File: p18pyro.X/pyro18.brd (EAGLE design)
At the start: 74.9 x 46.7 mm, 25 parts, among them U1 TPIC6B595PTH, U2 TPIC6B595PTH, X1 332-10, X2 332-10, X3 332-10, X4 332-10, X5 22-23-2041, X7 22-23-2021

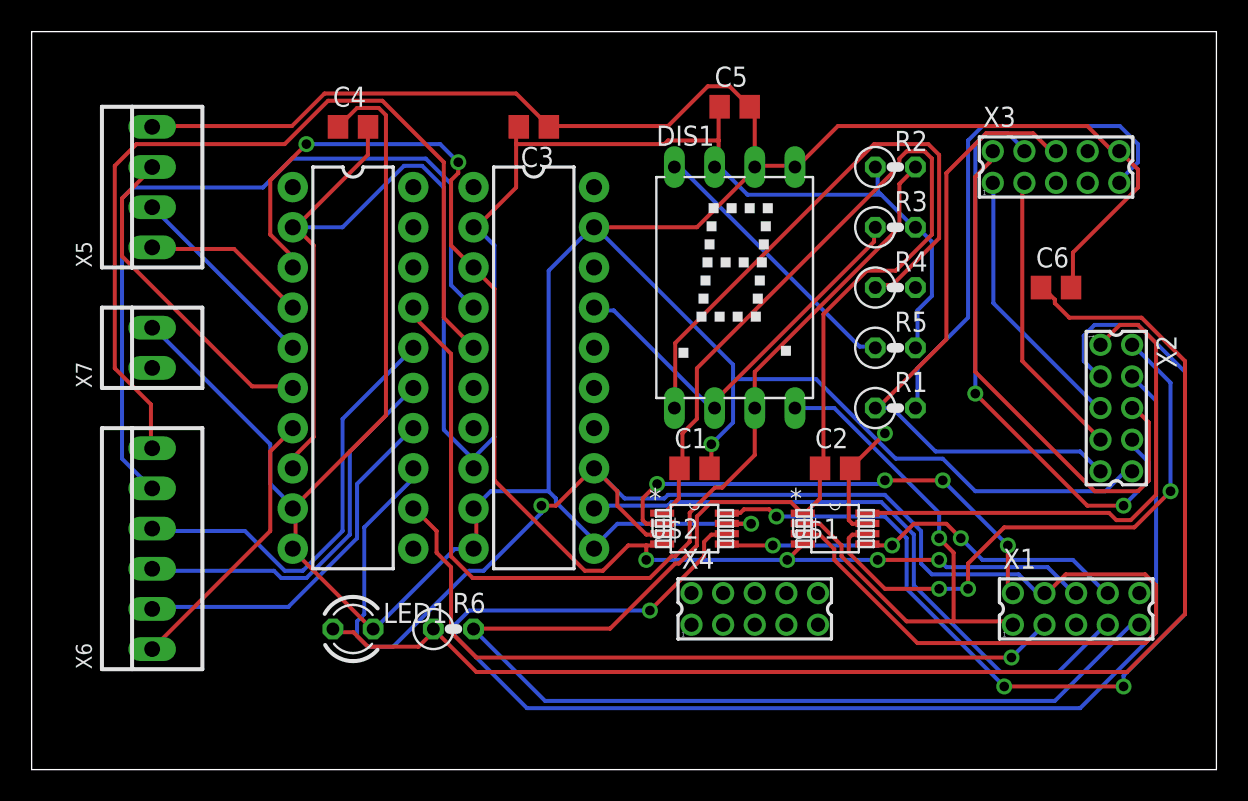
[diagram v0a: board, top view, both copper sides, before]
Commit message: update
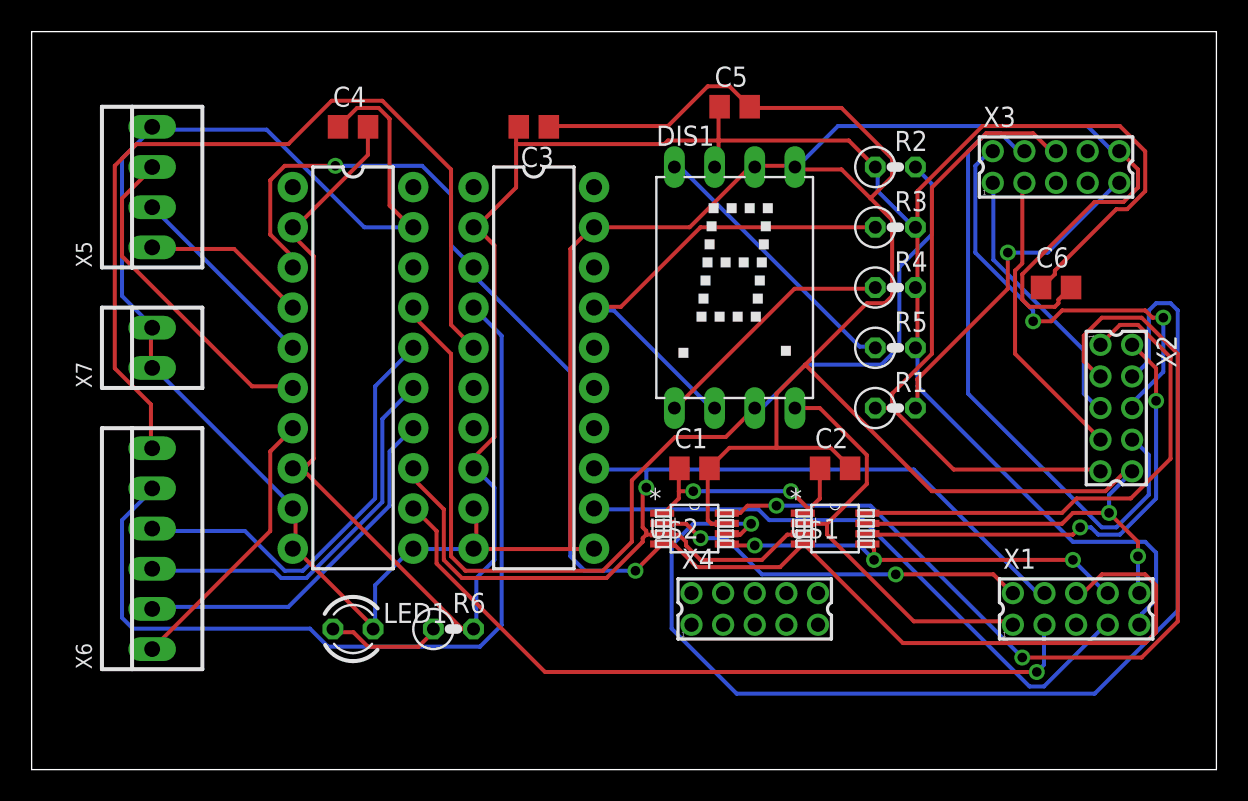
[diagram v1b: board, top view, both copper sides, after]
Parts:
- C1, C2, C3, C4, C5: value (none) -> 0.1
- C6: value (none) -> 22uf
- LED1: value (none) -> red
- R1: value (none) -> 662
- R2, R3, R4, R5, R6: value (none) -> 1k
- X6: value (none) -> out2 pins
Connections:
- removed net N$11: X7.1
- removed net N$5: U1.11
- removed net N$6: U1.19
- removed net VSS: X1.10
- net GND: now also U1.11, U1.19, X1.10, X7.1
- net N$35: no longer C6.1
- net VCC: now also C6.1, R4.2, R6.2, X1.9
- net VDD: no longer R6.2, X1.9
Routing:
- net VDD: track 129.6 -> 15.4 mm, vias 0 -> 2
- net N$35: track 84.7 -> 7.39 mm
- net VCC: track 121.0 -> 174.4 mm
- net N$7: track 108.7 -> 68.6 mm
- net GND: track 256.7 -> 283.6 mm, vias 3 -> 2
- net N$27: track 36.9 -> 15.9 mm
- net N$22: track 32.9 -> 21.2 mm, vias 0 -> 1
- net N$16: track 85.8 -> 74.4 mm
- net N$12: track 84.9 -> 95.7 mm, vias 6 -> 2
- net N$1: track 35.5 -> 27.5 mm, vias 1 -> 0
- net N$10: track 37.3 -> 29.9 mm, vias 3 -> 2
- net N$2: track 31.1 -> 24.0 mm, vias 4 -> 2
- net N$18: track 34.0 -> 28.1 mm, vias 0 -> 2
- net N$33: track 50.1 -> 55.1 mm
- net N$23: track 26.0 -> 30.2 mm
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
